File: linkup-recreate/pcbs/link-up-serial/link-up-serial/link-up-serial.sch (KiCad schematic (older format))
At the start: 10 parts

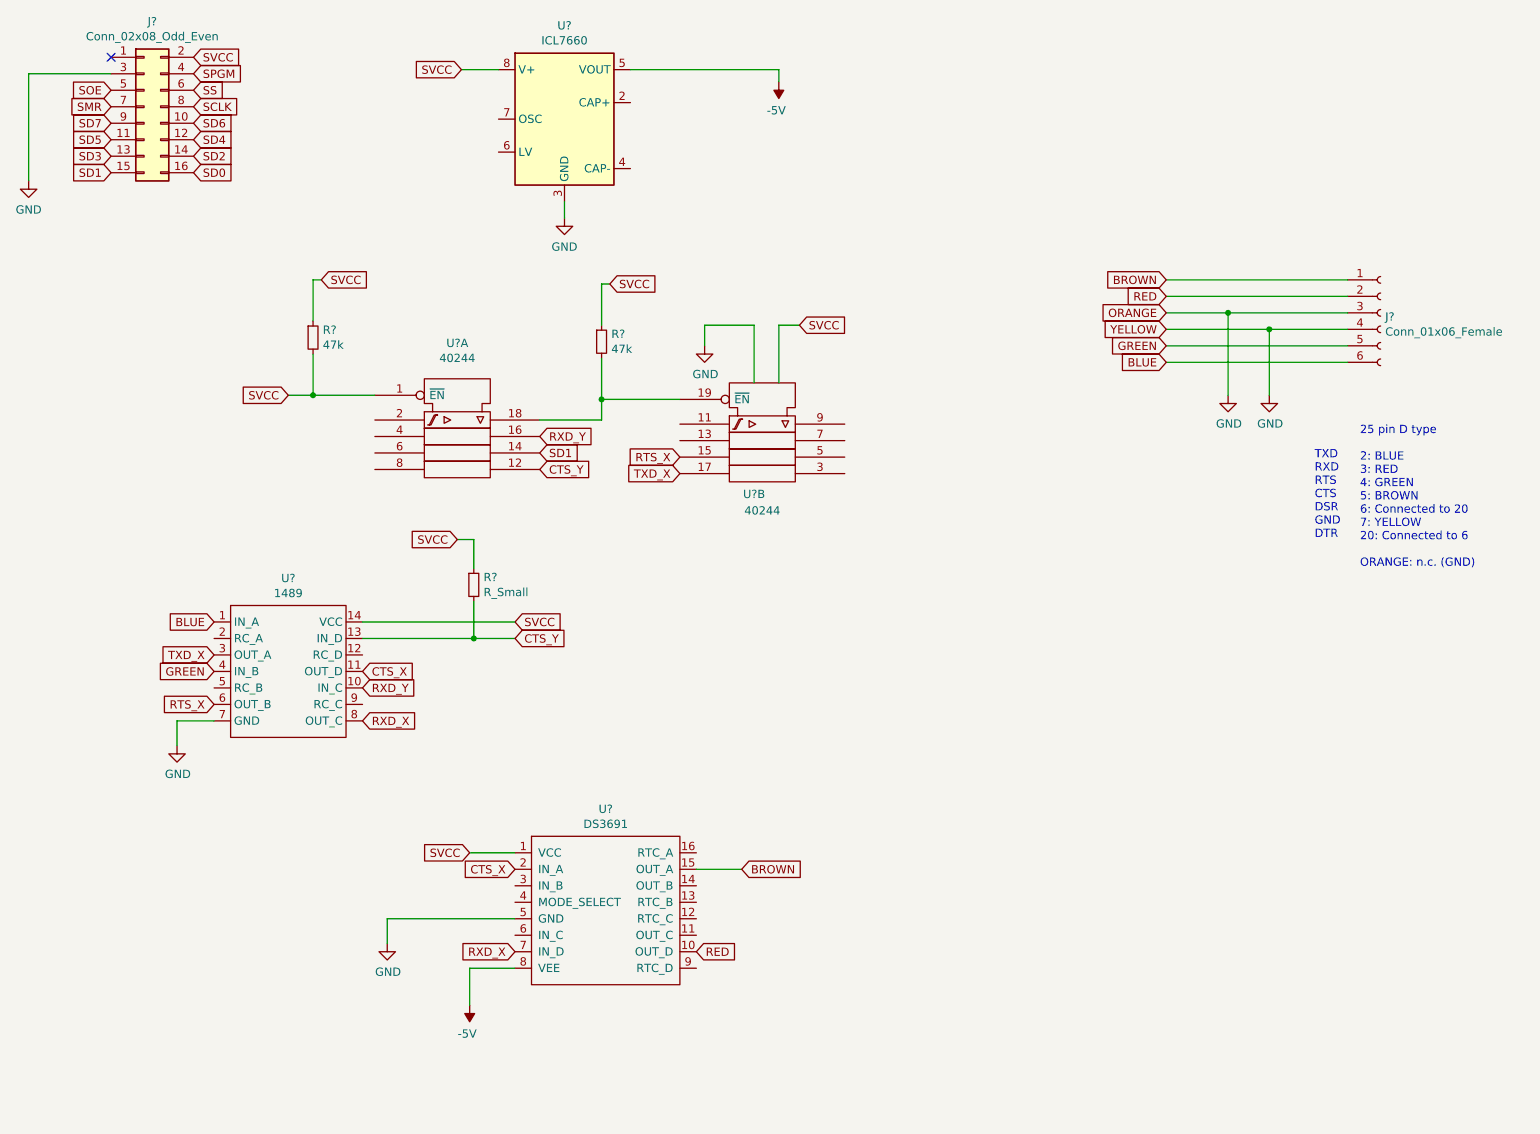
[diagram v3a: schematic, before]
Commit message: Updates
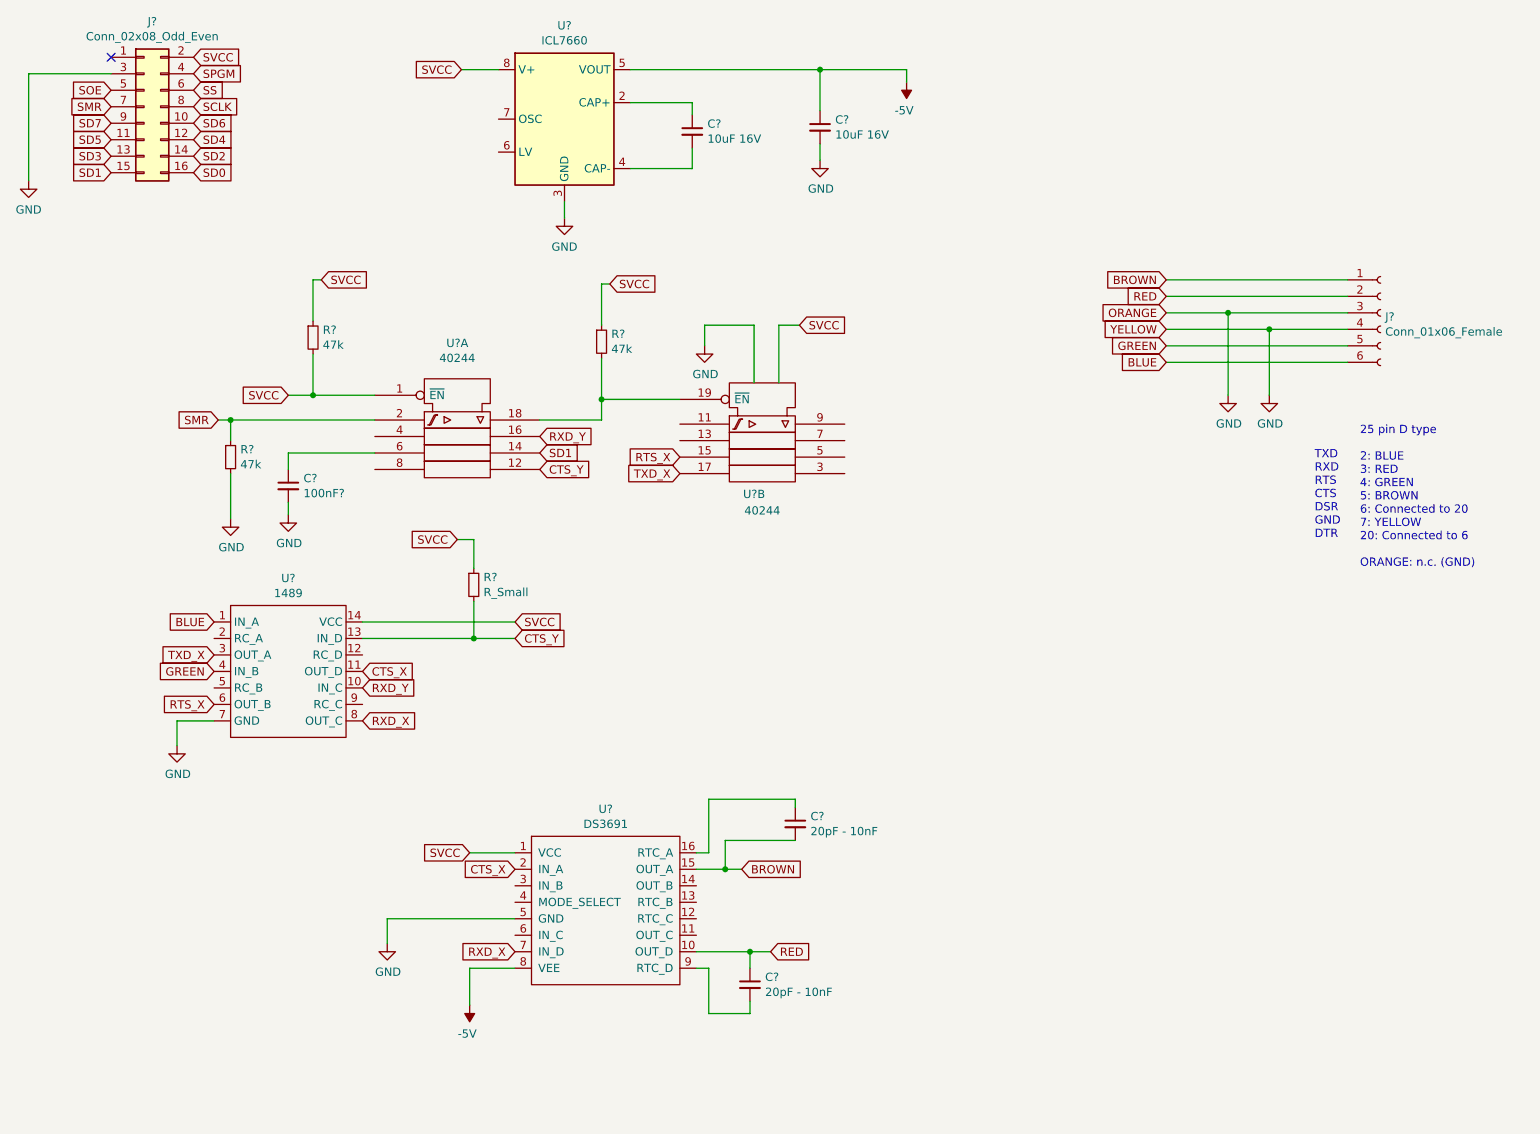
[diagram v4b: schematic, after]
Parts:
- added C? (x2): 10uF 16V, symbol Device:C_Small
- added C? (x2): 20pF - 10nF, symbol Device:C_Small
- added C?: 100nF?, symbol Device:C_Small
- added R?: 47k, symbol Device:R_Small
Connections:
- net -5V: now also C?.1
- net BROWN: now also C?.2
- net GND: now also C?.2, C?.2, R?.2
- net RED: now also C?.1
- net SMR: now also U?.2, R?.1
- net at U?.6: now also C?.1
- net at U?.16 (RTC_A): now also C?.1
- net at U?.9 (RTC_D): now also C?.2
- net at U?.2 (CAP+): now also C?.1
- net at U?.4 (CAP-): now also C?.2
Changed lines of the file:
@@
 L power:-5V #PWR?
 U 1 1 63721F90
-P 5525 1225
-F 0 "#PWR?" H 5525 1325 50  0001 C CNN
-F 1 "-5V" H 5540 1398 50  0000 C CNN
-F 2 "" H 5525 1225 50  0001 C CNN
-F 3 "" H 5525 1225 50  0001 C CNN
-	1    5525 1225
+P 6300 1225
+F 0 "#PWR?" H 6300 1325 50  0001 C CNN
+F 1 "-5V" H 6315 1398 50  0000 C CNN
+F 2 "" H 6300 1225 50  0001 C CNN
+F 3 "" H 6300 1225 50  0001 C CNN
+	1    6300 1225
 	-1   0    0    1
 $EndComp
@@
 	3650 6600 3650 6825
 Wire Wire Line
-	5525 1150 5525 1225
-Wire Wire Line
-	4625 1150 5525 1150
+	6300 1150 6300 1225
+Wire Wire Line
+	4625 1150 5775 1150
 Wire Wire Line
 	3925 5900 3650 5900
@@
 BROWN
 Wire Wire Line
-	5300 6000 5025 6000
+	5300 6000 5200 6000
 Text GLabel 4925 3600 0    50   Input ~ 0
 TXD_X
@@
 Text GLabel 3925 6500 0    50   Input ~ 0
 RXD_X
-Text GLabel 5025 6500 2    50   Input ~ 0
+Text GLabel 5475 6500 2    50   Input ~ 0
 RED
 Wire Wire Line
@@
 Wire Wire Line
 	3675 4600 3925 4600
+$Comp
+L Device:C_Small C?
+U 1 1 637349F7
+P 5000 1525
+F 0 "C?" H 5092 1571 50  0000 L CNN
+F 1 "10uF 16V" H 5092 1480 50  0000 L CNN
+F 2 "" H 5000 1525 50  0001 C CNN
+F 3 "~" H 5000 1525 50  0001 C CNN
+	1    5000 1525
+	1    0    0    -1
+$EndComp
+Wire Wire Line
+	4625 1350 5000 1350
+Wire Wire Line
+	5000 1350 5000 1425
+Wire Wire Line
+	4625 1750 5000 1750
+Wire Wire Line
+	5000 1750 5000 1625
+$Comp
+L Device:C_Small C?
+U 1 1 63738020
+P 5775 1500
+F 0 "C?" H 5867 1546 50  0000 L CNN
+F 1 "10uF 16V" H 5867 1455 50  0000 L CNN
+F 2 "" H 5775 1500 50  0001 C CNN
+F 3 "~" H 5775 1500 50  0001 C CNN
+	1    5775 1500
+	1    0    0    -1
+$EndComp
+Wire Wire Line
+	5775 1400 5775 1150
+Connection ~ 5775 1150
+Wire Wire Line
+	5775 1150 6300 1150
+$Comp
+L power:GND #PWR?
+U 1 1 637395A7
+P 5775 1700
+F 0 "#PWR?" H 5775 1450 50  0001 C CNN
+F 1 "GND" H 5780 1527 50  0000 C CNN
+F 2 "" H 5775 1700 50  0001 C CNN
+F 3 "" H 5775 1700 50  0001 C CNN
+	1    5775 1700
+	1    0    0    -1
+$EndComp
+Wire Wire Line
+	5775 1600 5775 1700
+$Comp
+L Device:C_Small C?
+U 1 1 6373AE6E
+P 5625 5725
+F 0 "C?" H 5717 5771 50  0000 L CNN
+F 1 "20pF - 10nF" H 5717 5680 50  0000 L CNN
+F 2 "" H 5625 5725 50  0001 C CNN
+F 3 "~" H 5625 5725 50  0001 C CNN
+	1    5625 5725
+	1    0    0    -1
+$EndComp
+Wire Wire Line
+	5025 5900 5100 5900
+Wire Wire Line
+	5100 5900 5100 5575
+Wire Wire Line
+	5100 5575 5625 5575
+Wire Wire Line
+	5625 5575 5625 5625
+Wire Wire Line
+	5625 5825 5200 5825
+Wire Wire Line
+	5200 5825 5200 6000
+Connection ~ 5200 6000
+Wire Wire Line
+	5200 6000 5025 6000
+Wire Wire Line
+	5475 6500 5350 6500
+$Comp
+L Device:C_Small C?
+U 1 1 6373EC72
+P 5350 6700
+F 0 "C?" H 5442 6746 50  0000 L CNN
+F 1 "20pF - 10nF" H 5442 6655 50  0000 L CNN
+F 2 "" H 5350 6700 50  0001 C CNN
+F 3 "~" H 5350 6700 50  0001 C CNN
+	1    5350 6700
+	1    0    0    -1
+$EndComp
+Wire Wire Line
+	5350 6600 5350 6500
+Connection ~ 5350 6500
+Wire Wire Line
+	5350 6500 5025 6500
+Wire Wire Line
+	5350 6800 5350 6875
+Wire Wire Line
+	5350 6875 5100 6875
+Wire Wire Line
+	5100 6875 5100 6600
+Wire Wire Line
+	5100 6600 5025 6600
+$Comp
+L Device:C_Small C?
+U 1 1 637424F4
+P 2550 3675
+F 0 "C?" H 2642 3721 50  0000 L CNN
+F 1 "100nF?" H 2642 3630 50  0000 L CNN
+F 2 "" H 2550 3675 50  0001 C CNN
+F 3 "~" H 2550 3675 50  0001 C CNN
+	1    2550 3675
+	1    0    0    -1
+$EndComp
+Wire Wire Line
+	2550 3575 2550 3475
+Wire Wire Line
+	2550 3475 3075 3475
+$Comp
+L power:GND #PWR?
+U 1 1 63745654
+P 2550 3850
+F 0 "#PWR?" H 2550 3600 50  0001 C CNN
+F 1 "GND" H 2555 3677 50  0000 C CNN
+F 2 "" H 2550 3850 50  0001 C CNN
+F 3 "" H 2550 3850 50  0001 C CNN
+	1    2550 3850
+	1    0    0    -1
+$EndComp
+Wire Wire Line
+	2550 3850 2550 3775
+Text GLabel 2125 3275 0    50   Input ~ 0
+SMR
+Wire Wire Line
+	2125 3275 2200 3275
+$Comp
+L Device:R_Small R?
+U 1 1 637491DA
+P 2200 3500
+F 0 "R?" H 2259 3546 50  0000 L CNN
+F 1 "47k" H 2259 3455 50  0000 L CNN
+F 2 "" H 2200 3500 50  0001 C CNN
+F 3 "~" H 2200 3500 50  0001 C CNN
+	1    2200 3500
+	1    0    0    -1
+$EndComp
+$Comp
+L power:GND #PWR?
+U 1 1 63749883
+P 2200 3875
+F 0 "#PWR?" H 2200 3625 50  0001 C CNN
+F 1 "GND" H 2205 3702 50  0000 C CNN
+F 2 "" H 2200 3875 50  0001 C CNN
+F 3 "" H 2200 3875 50  0001 C CNN
+	1    2200 3875
+	1    0    0    -1
+$EndComp
+Wire Wire Line
+	2200 3875 2200 3600
+Wire Wire Line
+	2200 3400 2200 3275
+Connection ~ 2200 3275
+Wire Wire Line
+	2200 3275 3075 3275
 $EndSCHEMATC

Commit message: Updates
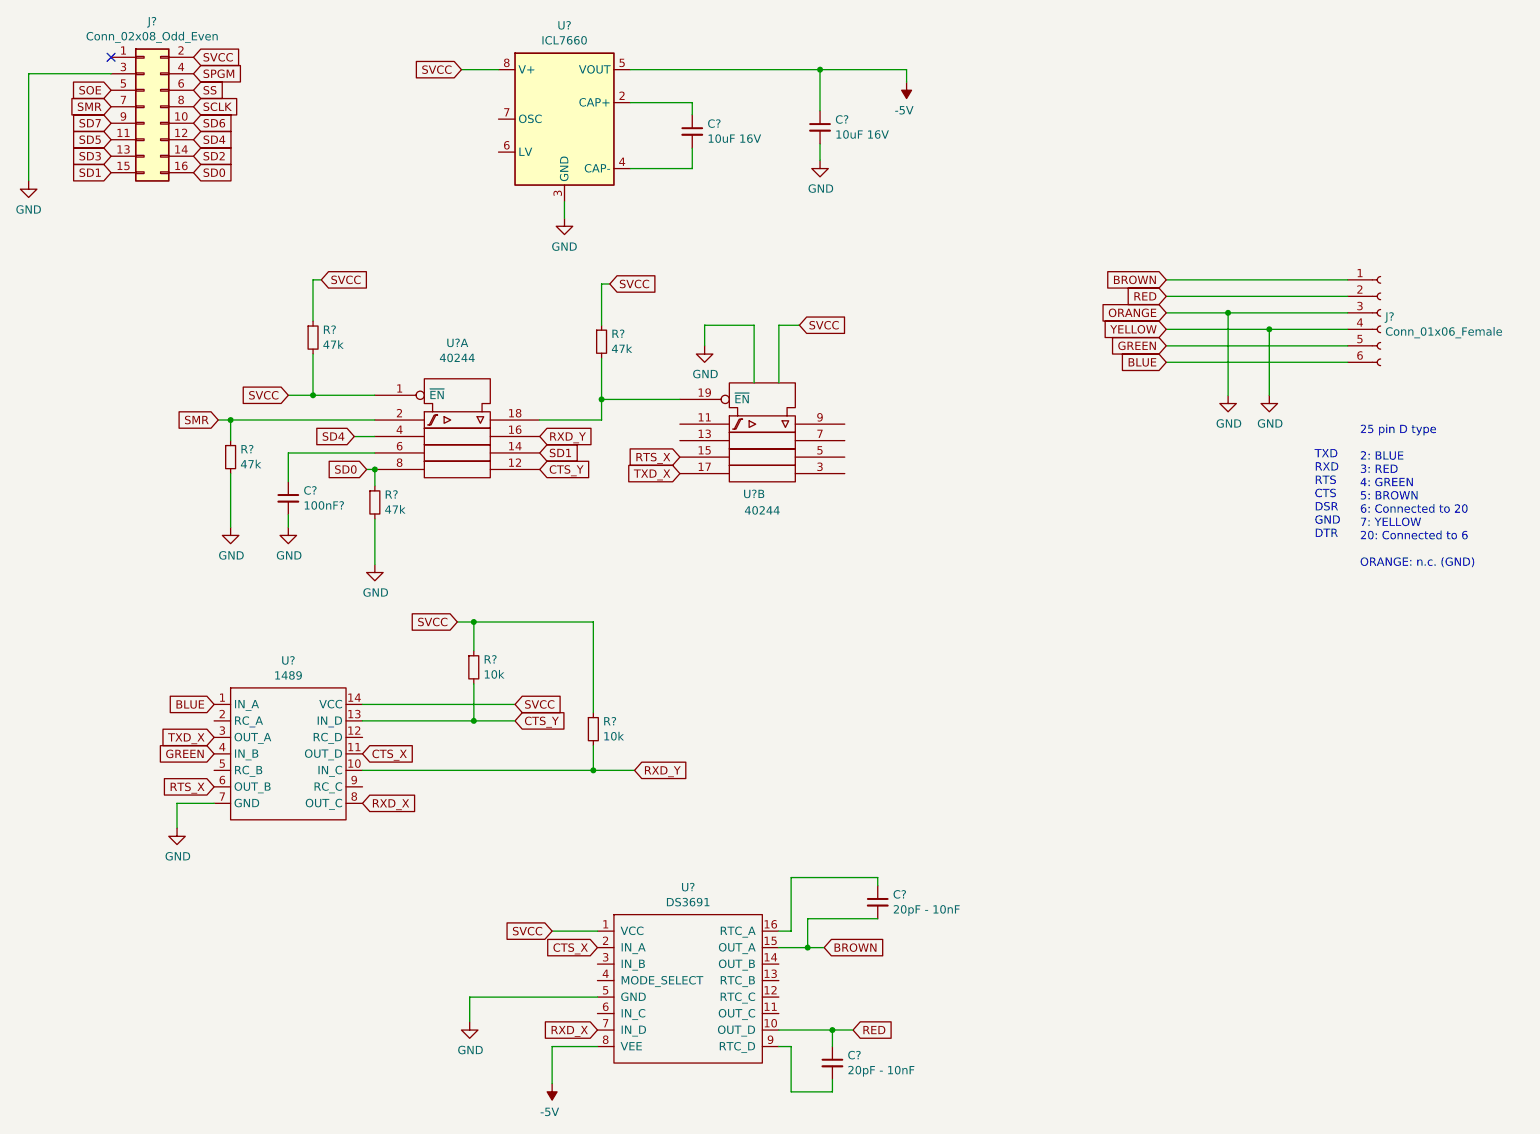
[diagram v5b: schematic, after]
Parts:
- added R?: 10k, symbol Device:R_Small
- added R?: 47k, symbol Device:R_Small
- R?: value R_Small -> 10k
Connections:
- net GND: now also R?.2
- net RXD_Y: now also R?.2
- net SD0: now also U?.8, R?.1
- net SD4: now also U?.4
- net Vdd: now also R?.1
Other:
- moved on the sheet: C?, R?, U?

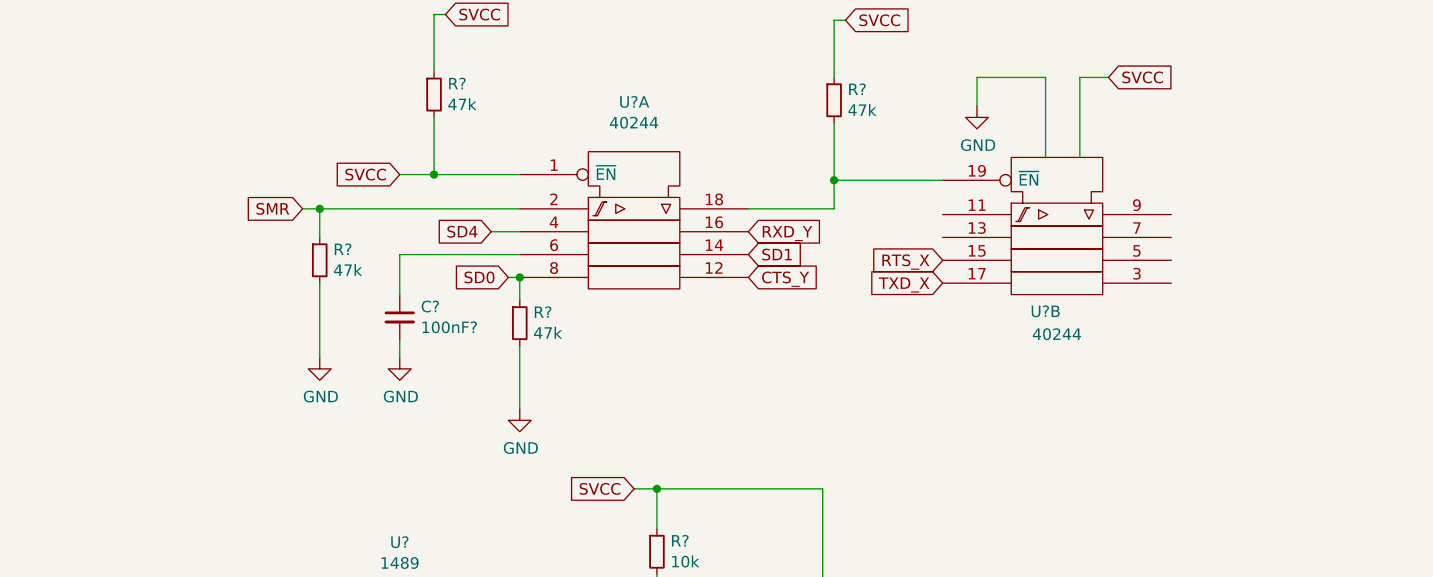
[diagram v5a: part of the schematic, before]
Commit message: Updates
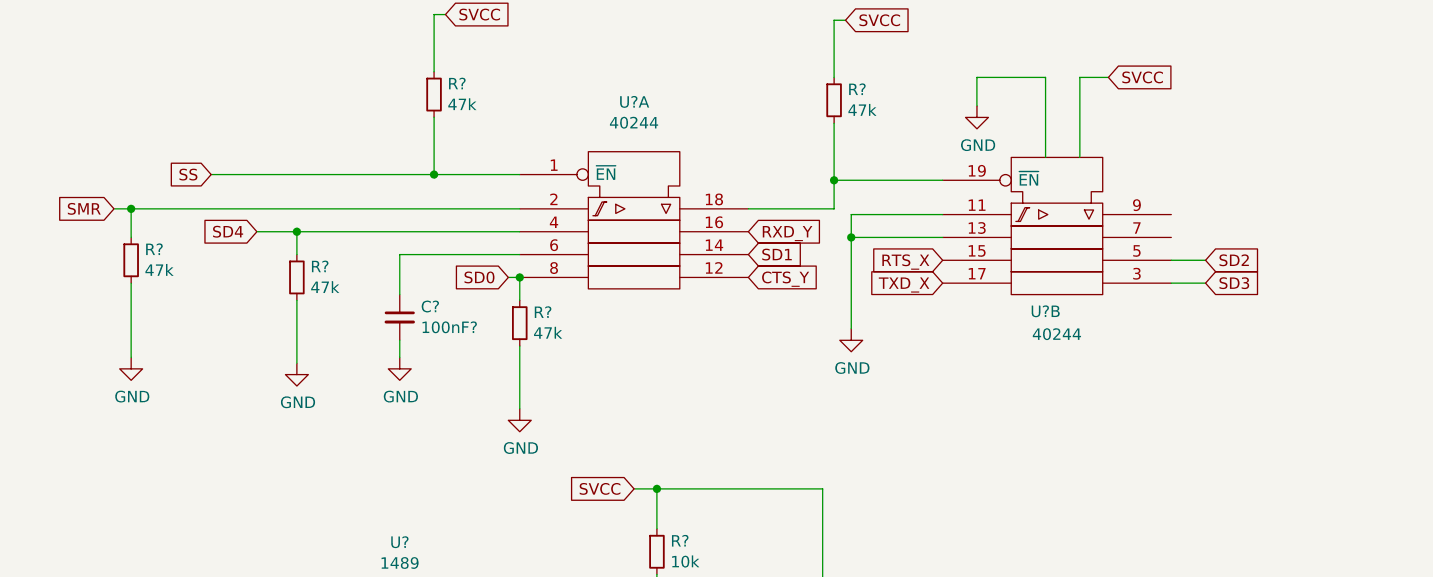
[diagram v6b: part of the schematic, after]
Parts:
- added R?: 47k, symbol Device:R_Small
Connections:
- net GND: now also U?.11, U?.13, R?.2
- net SD2: now also U?.5
- net SD3: now also U?.3
- net SD4: now also R?.1
- net SS: now also R?.2, U?.1 (~EN)
- net Vdd: no longer R?.2, U?.1 (~EN)
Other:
- moved on the sheet: R?
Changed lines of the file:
@@
 	1    0    0    -1
 $EndComp
-Text GLabel 2550 3125 0    50   Input ~ 0
-SVCC
-Wire Wire Line
-	2550 3125 2700 3125
+Text GLabel 1725 3125 0    50   Input ~ 0
+SS
+Wire Wire Line
+	1725 3125 2700 3125
 Wire Wire Line
 	2700 2875 2700 3125
@@
 Wire Wire Line
 	2550 3925 2550 3850
-Text GLabel 2125 3275 0    50   Input ~ 0
+Text GLabel 1300 3275 0    50   Input ~ 0
 SMR
 Wire Wire Line
-	2125 3275 2200 3275
+	1300 3275 1375 3275
 $Comp
 L Device:R_Small R?
 U 1 1 637491DA
-P 2200 3500
-F 0 "R?" H 2259 3546 50  0000 L CNN
-F 1 "47k" H 2259 3455 50  0000 L CNN
-F 2 "" H 2200 3500 50  0001 C CNN
-F 3 "~" H 2200 3500 50  0001 C CNN
-	1    2200 3500
+P 1375 3500
+F 0 "R?" H 1434 3546 50  0000 L CNN
+F 1 "47k" H 1434 3455 50  0000 L CNN
+F 2 "" H 1375 3500 50  0001 C CNN
+F 3 "~" H 1375 3500 50  0001 C CNN
+	1    1375 3500
 	1    0    0    -1
 $EndComp
@@
 L power:GND #PWR?
 U 1 1 63749883
-P 2200 3925
-F 0 "#PWR?" H 2200 3675 50  0001 C CNN
-F 1 "GND" H 2205 3752 50  0000 C CNN
-F 2 "" H 2200 3925 50  0001 C CNN
-F 3 "" H 2200 3925 50  0001 C CNN
-	1    2200 3925
-	1    0    0    -1
-$EndComp
-Wire Wire Line
-	2200 3925 2200 3600
-Wire Wire Line
-	2200 3400 2200 3275
-Connection ~ 2200 3275
-Wire Wire Line
-	2200 3275 3075 3275
-Text GLabel 2950 3375 0    50   Input ~ 0
+P 1375 3925
+F 0 "#PWR?" H 1375 3675 50  0001 C CNN
+F 1 "GND" H 1380 3752 50  0000 C CNN
+F 2 "" H 1375 3925 50  0001 C CNN
+F 3 "" H 1375 3925 50  0001 C CNN
+	1    1375 3925
+	1    0    0    -1
+$EndComp
+Wire Wire Line
+	1375 3925 1375 3600
+Wire Wire Line
+	1375 3400 1375 3275
+Connection ~ 1375 3275
+Wire Wire Line
+	1375 3275 3075 3275
+Text GLabel 1925 3375 0    50   Input ~ 0
 SD4
-Wire Wire Line
-	2950 3375 3075 3375
 $Comp
 L Device:R_Small R?
@@
 	3025 3575 3075 3575
 Connection ~ 3075 3575
+Wire Wire Line
+	1925 3375 2100 3375
+$Comp
+L Device:R_Small R?
+U 1 1 6377586C
+P 2100 3575
+F 0 "R?" H 2159 3621 50  0000 L CNN
+F 1 "47k" H 2159 3530 50  0000 L CNN
+F 2 "" H 2100 3575 50  0001 C CNN
+F 3 "~" H 2100 3575 50  0001 C CNN
+	1    2100 3575
+	1    0    0    -1
+$EndComp
+$Comp
+L power:GND #PWR?
+U 1 1 63775872
+P 2100 3950
+F 0 "#PWR?" H 2100 3700 50  0001 C CNN
+F 1 "GND" H 2105 3777 50  0000 C CNN
+F 2 "" H 2100 3950 50  0001 C CNN
+F 3 "" H 2100 3950 50  0001 C CNN
+	1    2100 3950
+	1    0    0    -1
+$EndComp
+Wire Wire Line
+	2100 3950 2100 3675
+Wire Wire Line
+	2100 3475 2100 3375
+Connection ~ 2100 3375
+Wire Wire Line
+	2100 3375 3075 3375
+Text GLabel 6075 3600 2    50   Input ~ 0
+SD3
+Wire Wire Line
+	6075 3600 5925 3600
+Text GLabel 6075 3500 2    50   Input ~ 0
+SD2
+Wire Wire Line
+	6075 3500 5925 3500
+$Comp
+L power:GND #PWR?
+U 1 1 6377FAA5
+P 4525 3800
+F 0 "#PWR?" H 4525 3550 50  0001 C CNN
+F 1 "GND" H 4530 3627 50  0000 C CNN
+F 2 "" H 4525 3800 50  0001 C CNN
+F 3 "" H 4525 3800 50  0001 C CNN
+	1    4525 3800
+	1    0    0    -1
+$EndComp
+Wire Wire Line
+	4925 3300 4525 3300
+Wire Wire Line
+	4525 3300 4525 3400
+Wire Wire Line
+	4925 3400 4525 3400
+Connection ~ 4525 3400
+Wire Wire Line
+	4525 3400 4525 3800
 $EndSCHEMATC
